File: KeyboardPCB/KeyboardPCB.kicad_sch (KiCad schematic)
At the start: 0 parts

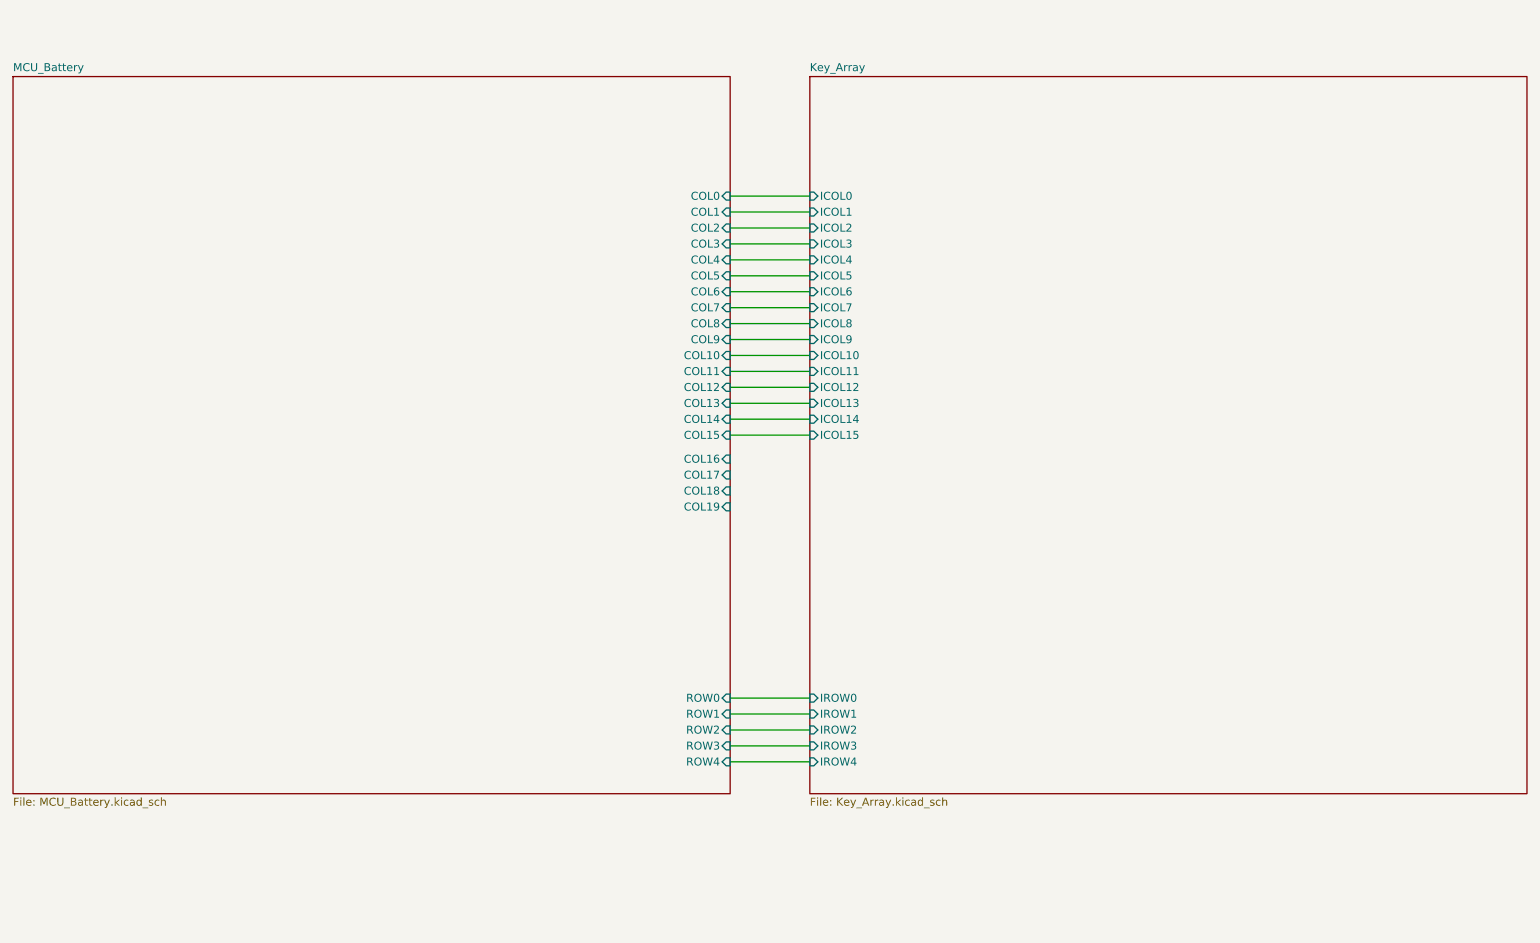
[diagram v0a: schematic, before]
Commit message: reorganised the schematic
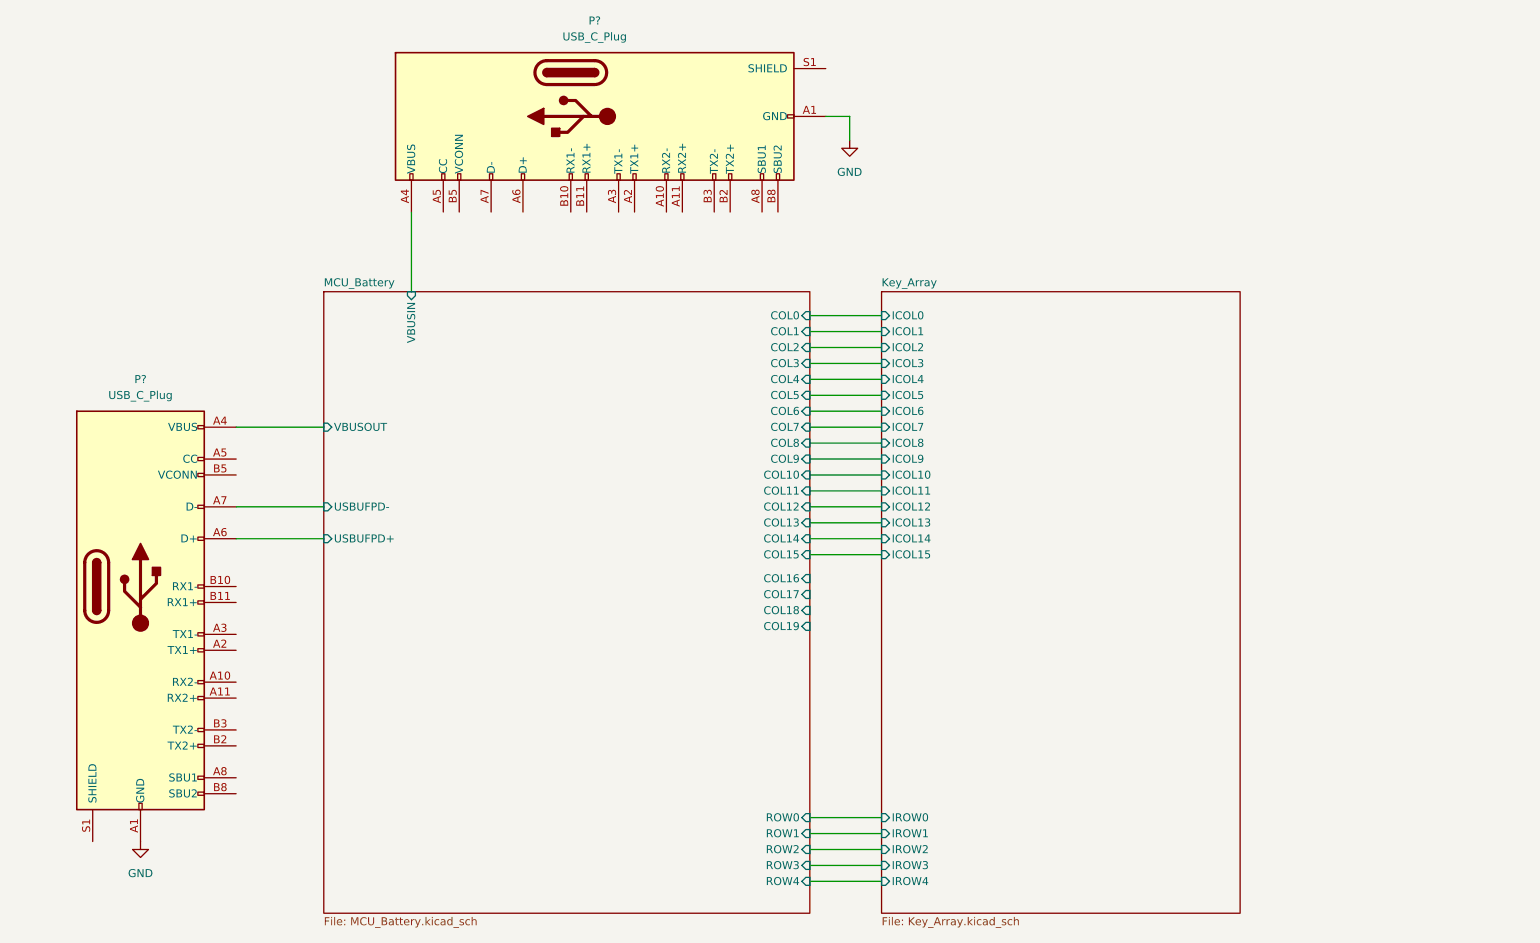
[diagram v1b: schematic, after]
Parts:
- added P? (x2): USB_C_Plug, symbol Connector:USB_C_Plug
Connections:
- new net GND: P?.A1 (GND), P?.A1 (GND), P?.A12 (GND), P?.A12 (GND), P?.B1 (GND), P?.B1 (GND), P?.B12 (GND), P?.B12 (GND)
- new net MCU_Battery/USBUFPD+: P?.A6 (D+)
- new net MCU_Battery/USBUFPD-: P?.A7 (D-)
- new net MCU_Battery/VBUSIN: P?.A4 (VBUS), P?.A9 (VBUS), P?.B4 (VBUS), P?.B9 (VBUS)
- new net MCU_Battery/VBUSOUT: P?.A4 (VBUS), P?.A9 (VBUS), P?.B4 (VBUS), P?.B9 (VBUS)
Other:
- sheet MCU_Battery ports: added USBUFPD+, USBUFPD-, VBUSIN, VBUSOUT; removed none
